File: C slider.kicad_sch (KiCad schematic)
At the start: 2 parts, among them U1 ESP32-S3-WROOM-1-N8R8

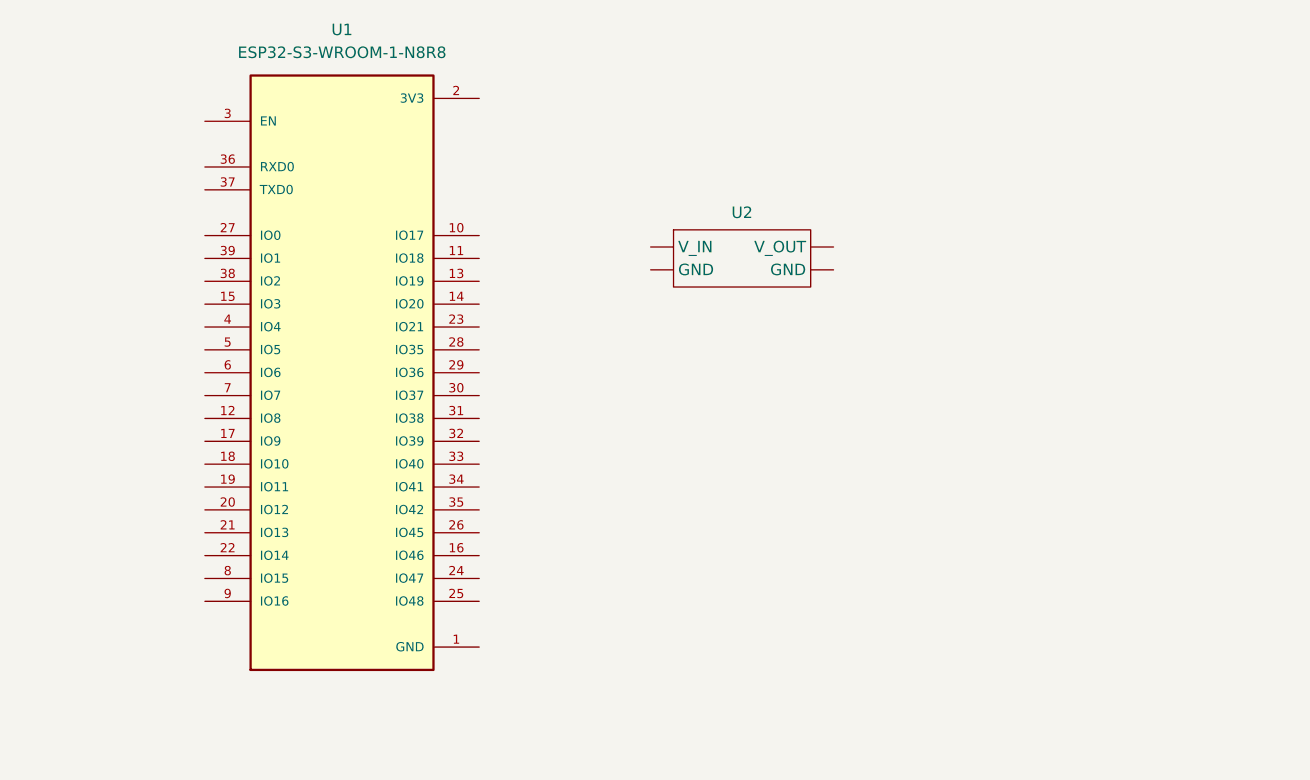
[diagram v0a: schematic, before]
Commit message: vytvoreni schemy a desky
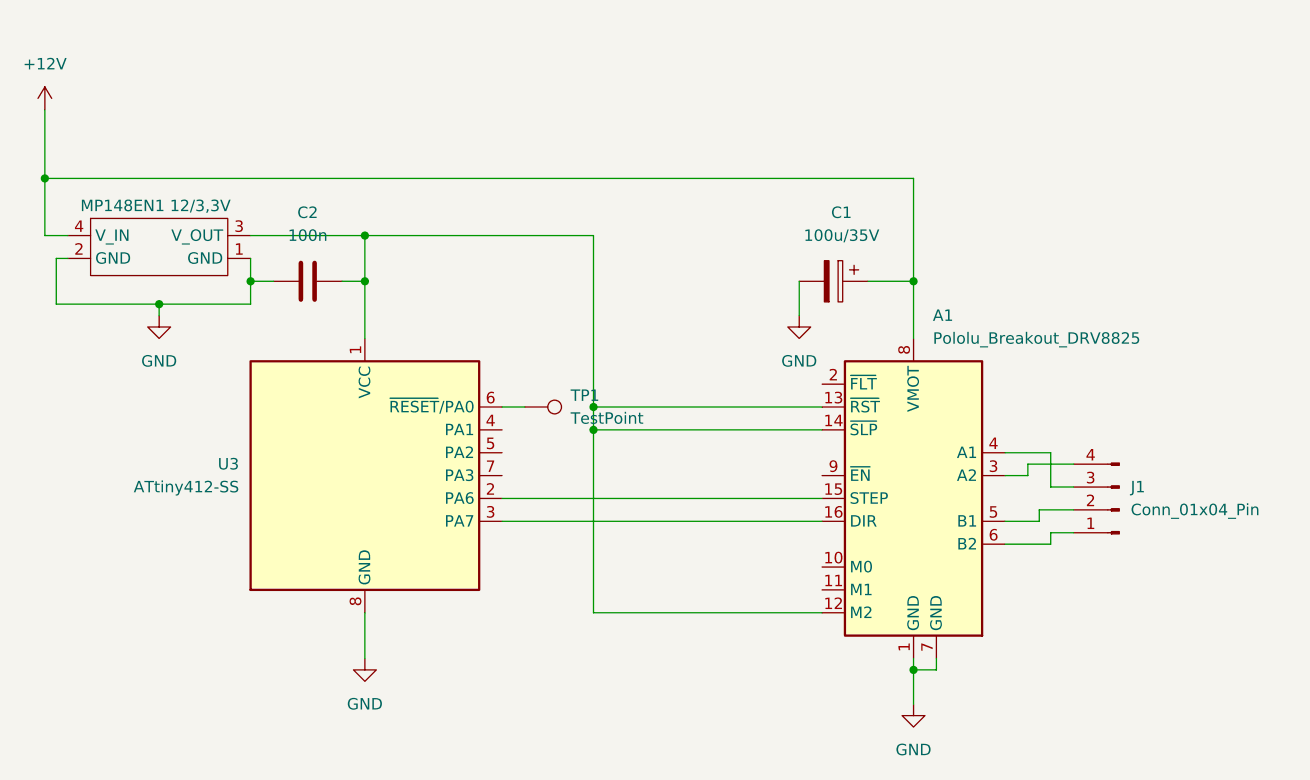
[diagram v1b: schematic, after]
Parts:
- removed U1: ESP32-S3-WROOM-1-N8R8, ESP32-S3-WROOM-1-N8R8:XCVR_ESP32S3WROOM1N8R8, symbol ESP32-S3-WROOM-1-N8R8:ESP32-S3-WROOM-1-N8R8
- removed U2: (no value), ESP32-S3-WROOM-1-N8R8:XCVR_ESP32S3WROOM1N8R8, symbol Moduly:Stepdown_DC/DC
- added A1: Pololu_Breakout_DRV8825, Module:Pololu_Breakout-16_15.2x20.3mm, symbol Driver_Motor:Pololu_Breakout_DRV8825
- added C1: 100u/35V, Capacitor_THT:CP_Radial_D8.0mm_P3.80mm, symbol Device:C_Polarized
- added C2: 100n, Capacitor_THT:C_Disc_D3.0mm_W1.6mm_P2.50mm, symbol Device:C
- added J1: Conn_01x04_Pin, Connector_PinHeader_2.54mm:PinHeader_1x04_P2.54mm_Vertical, symbol Connector:Conn_01x04_Pin
- added MP148EN1: 12/3,3V, StepDown:MP148EN1, symbol Moduly:Stepdown_DC/DC
- added TP1: TestPoint, TestPoint:TestPoint_Pad_D2.0mm, symbol Connector:TestPoint
- added U3: ATtiny412-SS, Package_SO:SOIC-8_3.9x4.9mm_P1.27mm, symbol MCU_Microchip_ATtiny:ATtiny412-SS
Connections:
- net GND: now also A1.1 (GND), A1.7 (GND), C1.2, C2.1, MP148EN1.1 (GND), MP148EN1.2 (GND), U3.8 (GND)
- new net: A1.12 (M2), A1.13 (~{RST}), A1.14 (~{SLP}), C2.2, MP148EN1.3 (V_OUT), U3.1 (VCC)
- new net: A1.15 (STEP), U3.2 (PA6)
- new net: A1.16 (DIR), U3.3 (PA7)
- new net: TP1.1, U3.6 (~{RESET}/PA0)
- new net: A1.3 (A2), J1.4 (Pin_4)
- new net: A1.4 (A1), J1.3 (Pin_3)
- new net: A1.5 (B1), J1.2 (Pin_2)
- new net: A1.6 (B2), J1.1 (Pin_1)
- new net +12V: A1.8 (VMOT), C1.1, MP148EN1.4 (V_IN)
